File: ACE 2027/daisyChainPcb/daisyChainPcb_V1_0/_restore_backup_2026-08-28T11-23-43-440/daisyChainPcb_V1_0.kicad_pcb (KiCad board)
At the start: 2 copper layers, 56.5 x 97 mm, 26 parts, among them J201 Pads, J202 XT30, J203 XT30, J204 Pads, J205 Pads, J206 RJ45, J207 RJ45, U101 AP7361C-33E-13

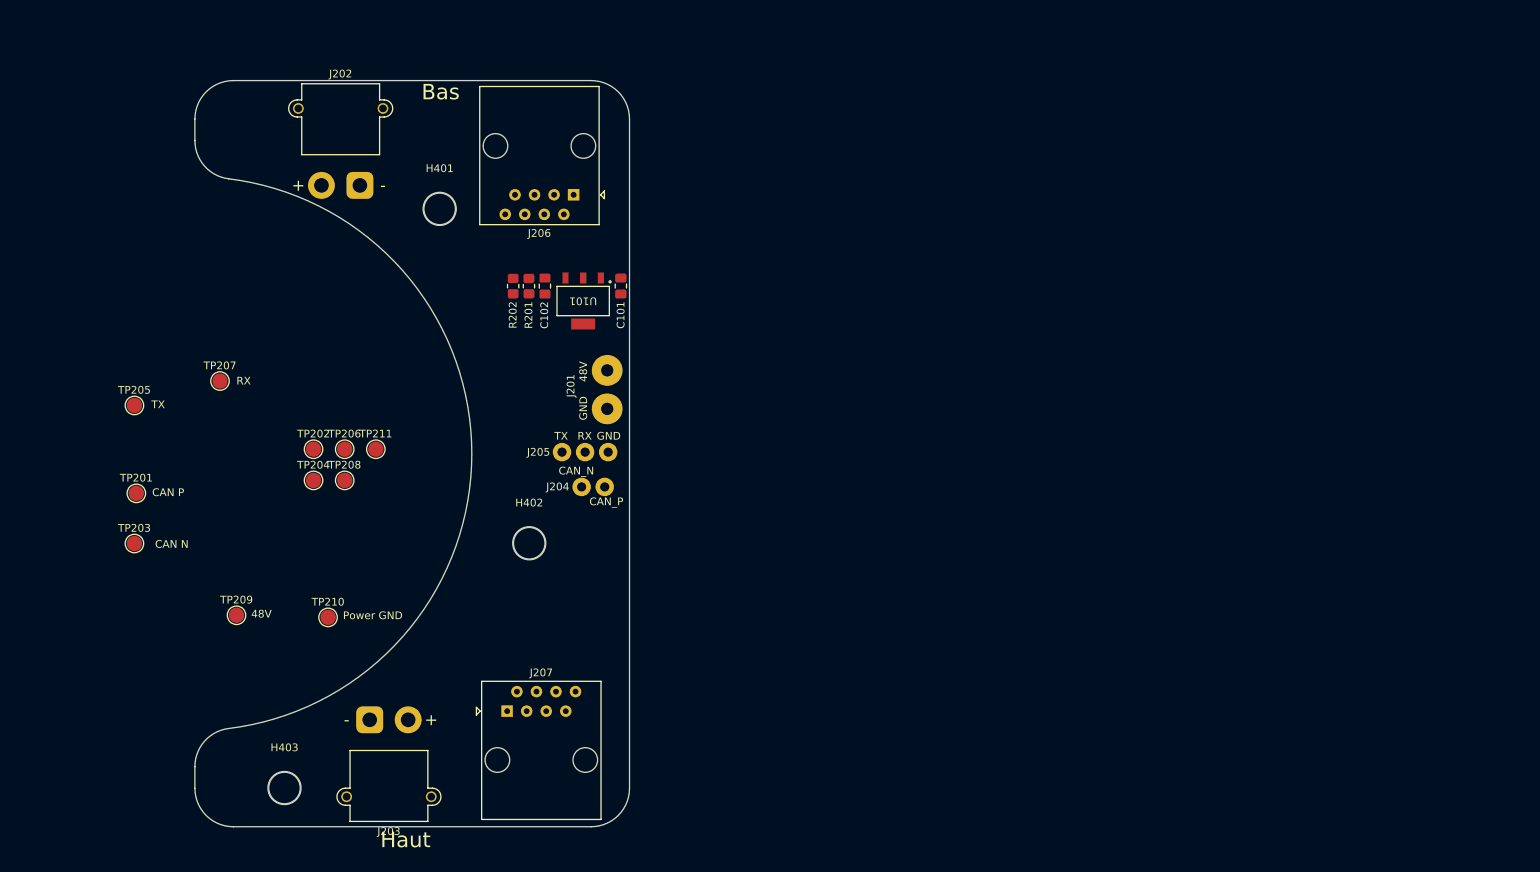
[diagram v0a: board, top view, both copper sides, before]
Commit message: Saving before trying a new layout
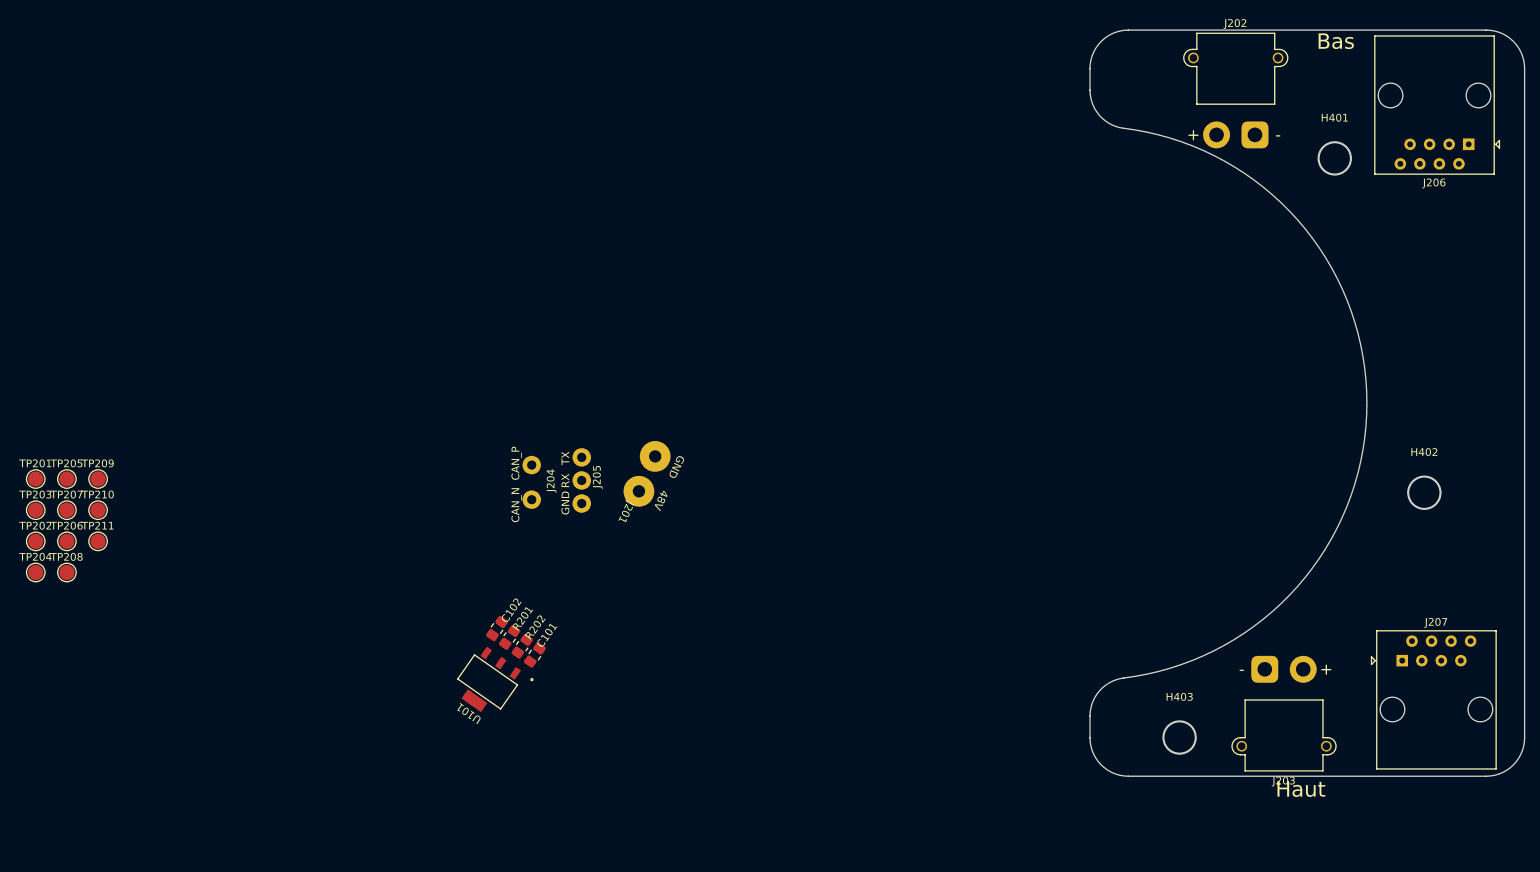
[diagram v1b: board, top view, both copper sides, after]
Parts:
- moved H401 116.5 mm to (257.9, 49.1)
- moved J202 116.5 mm to (247.5, 46.1)
- moved J203 116.5 mm to (248.8, 115.5)
- moved J206 116.5 mm to (275.3, 47.3)
- moved J207 116.5 mm to (266.7, 114.4)
- moved H403 116.5 mm to (237.7, 124.4)
- moved H402 116.5 mm to (269.5, 92.6)
- moved U101 51.1 mm to (147.8, 117.2), turned to 145 degrees
- moved C101 49.3 mm to (153.9, 113.7), turned to 55 degrees
- moved R202 46.8 mm to (152.3, 112.5), turned to -125 degrees
- moved R201 45.7 mm to (150.6, 111.4), turned to -125 degrees
- moved C102 44.9 mm to (149.0, 110.3), turned to 55 degrees
- moved TP211 38.0 mm to (97.1, 98.9)
- moved TP202 38.0 mm to (89.0, 98.9)
- moved TP204 38.0 mm to (89.0, 103.0)
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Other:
- board text removed: "48V"
- board text removed: "CAN N"
- board text removed: "CAN P"
- board text removed: "Power GND"
- board text removed: "RX"
- board text removed: "TX"
